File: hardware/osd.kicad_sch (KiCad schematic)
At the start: 21 parts, among them U10 COS8051SOT, U11 TLV7031DPWR, U18 SN74LVC1G3157DTBR

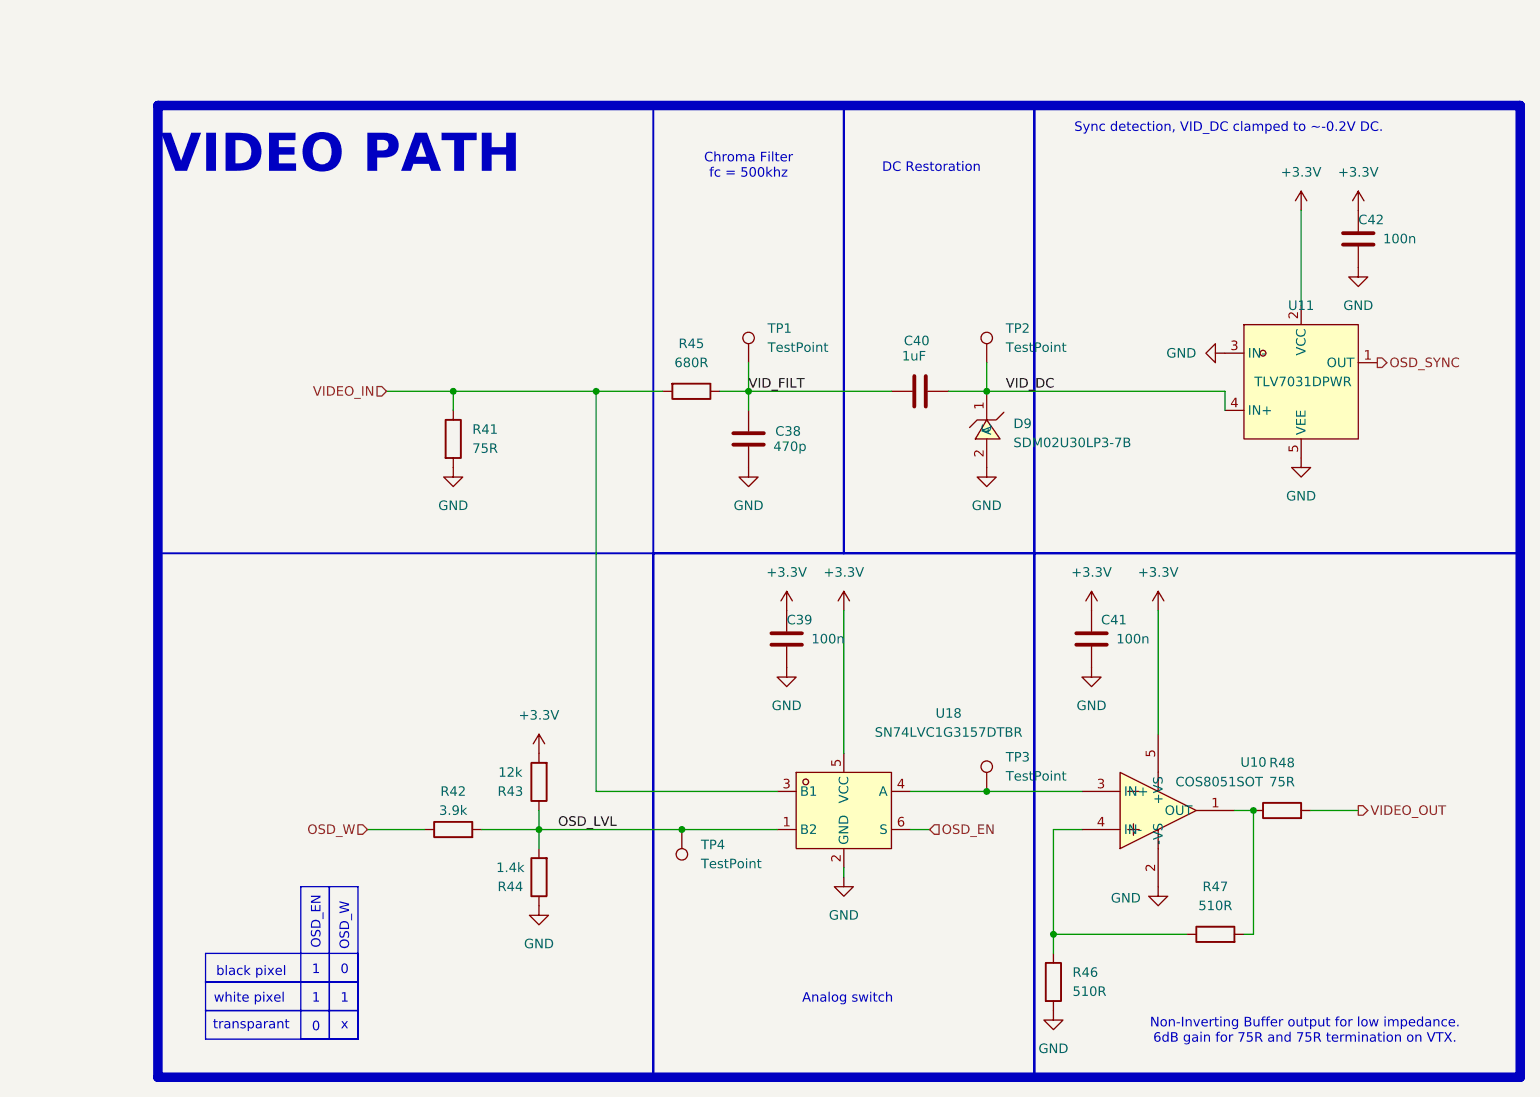
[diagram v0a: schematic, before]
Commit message: routing
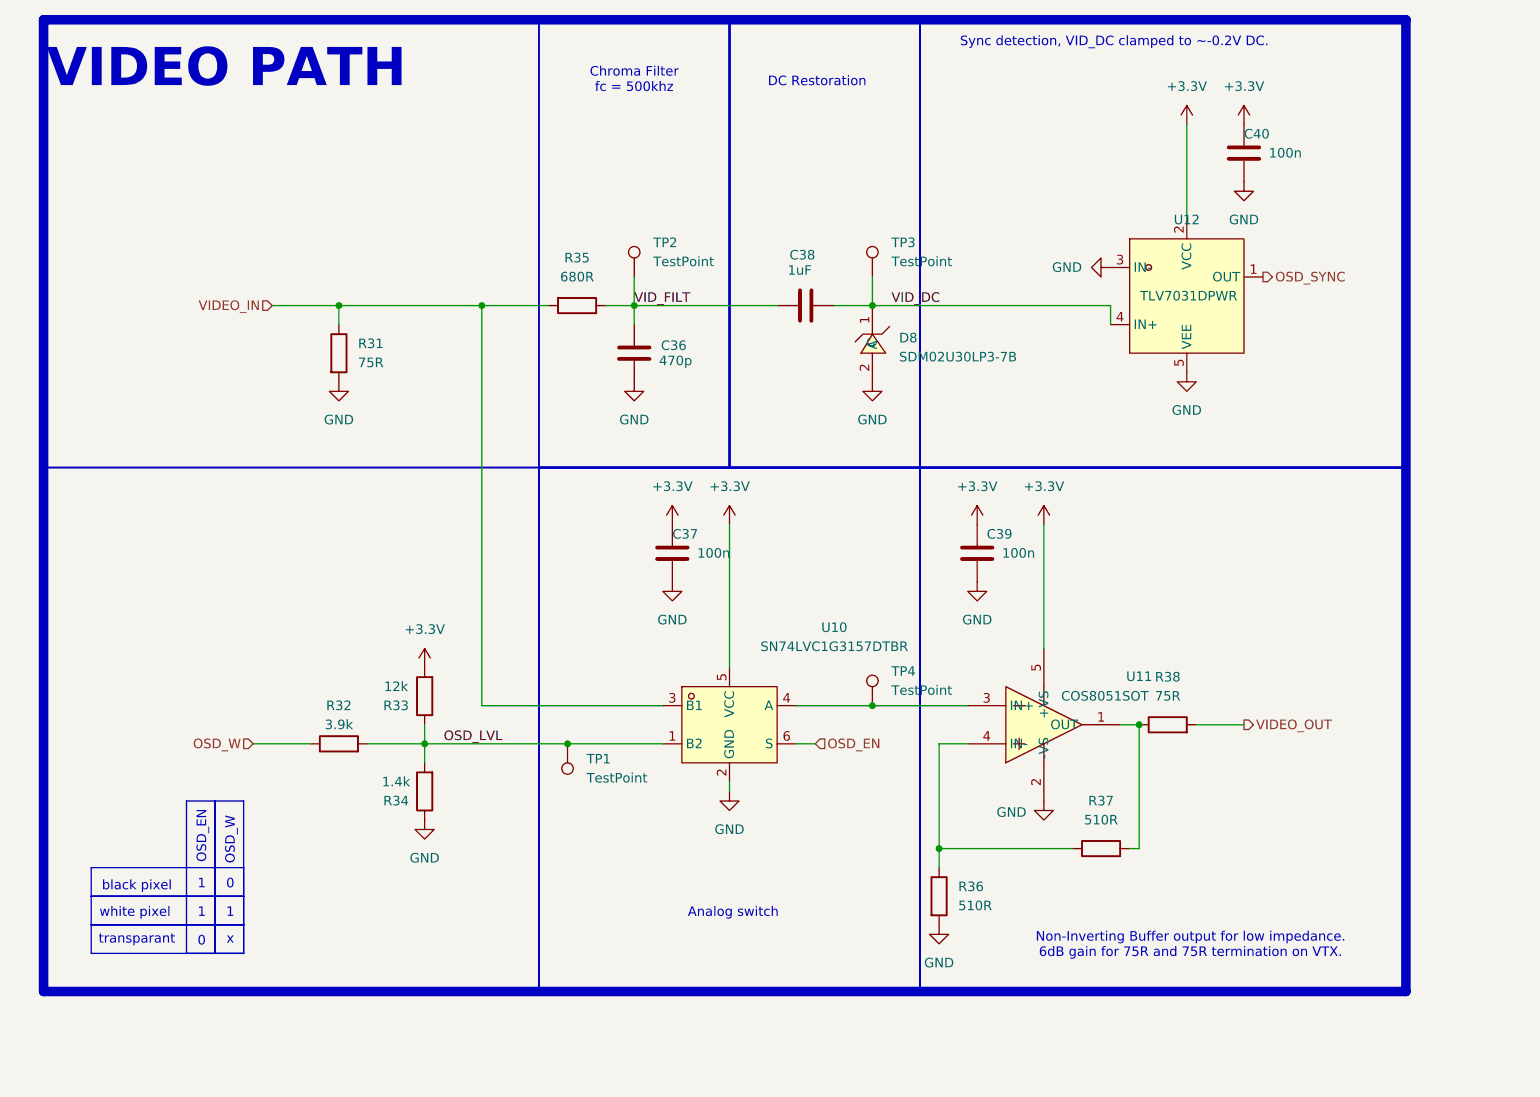
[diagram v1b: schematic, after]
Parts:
- removed C41, C42: 100n, Capacitor_SMD:C_0201_0603Metric, symbol Device:C
- removed D9: SDM02U30LP3-7B, lib:X3-DFN0603-2_L0.6-W0.3-RD, symbol lib:SDM02U30LP3-7B
- removed R41, R48: 75R, Resistor_SMD:R_0201_0603Metric, symbol Device:R
- removed R42: 3.9k, Resistor_SMD:R_0201_0603Metric, symbol Device:R
- removed R43: 12k, Resistor_SMD:R_0201_0603Metric, symbol Device:R
- removed R44: 1.4k, Resistor_SMD:R_0201_0603Metric, symbol Device:R
- removed R45: 680R, Resistor_SMD:R_0201_0603Metric, symbol Device:R
- removed R46, R47: 510R, Resistor_SMD:R_0201_0603Metric, symbol Device:R
- removed U10: COS8051SOT, lib:SOT-23-5_L3.0-W1.7-P0.95-LS2.8-BR, symbol lib:COS8051SOT
- removed U11: TLV7031DPWR, lib:X2SON-4_L0.8-W0.8-P0.48-TL-A, symbol lib:TLV7031DPWR
- removed U18: SN74LVC1G3157DTBR, lib:X2SON-6_L1.0-W0.8-BL, symbol lib:SN74LVC1G3157DTBR
- added C36: 470p, Capacitor_SMD:C_0201_0603Metric, symbol Device:C
- added C37: 100n, Capacitor_SMD:C_0201_0603Metric, symbol Device:C
- added D8: SDM02U30LP3-7B, lib:X3-DFN0603-2_L0.6-W0.3-RD, symbol lib:SDM02U30LP3-7B
- added R31, R38: 75R, Resistor_SMD:R_0201_0603Metric, symbol Device:R
- added R32: 3.9k, Resistor_SMD:R_0201_0603Metric, symbol Device:R
- added R33: 12k, Resistor_SMD:R_0201_0603Metric, symbol Device:R
- added R34: 1.4k, Resistor_SMD:R_0201_0603Metric, symbol Device:R
- added R35: 680R, Resistor_SMD:R_0201_0603Metric, symbol Device:R
- added R36, R37: 510R, Resistor_SMD:R_0201_0603Metric, symbol Device:R
- added U10: SN74LVC1G3157DTBR, lib:X2SON-6_L1.0-W0.8-BL, symbol lib:SN74LVC1G3157DTBR
- added U11: COS8051SOT, lib:SOT-23-5_L3.0-W1.7-P0.95-LS2.8-BR, symbol lib:COS8051SOT
- added U12: TLV7031DPWR, lib:X2SON-4_L0.8-W0.8-P0.48-TL-A, symbol lib:TLV7031DPWR
- C38: value 470p -> 1uF; footprint Capacitor_SMD:C_0201_0603Metric -> Capacitor_SMD:C_0402_1005Metric; LCSC C526944 -> C52923; MPN CC0201JRX7R9BB471 -> CL05A105KA5NQNC; Manufacturer YAGEO -> Samsung Electro-Mechanics
- C40: value 1uF -> 100n; footprint Capacitor_SMD:C_0402_1005Metric -> Capacitor_SMD:C_0201_0603Metric; LCSC C52923 -> C76928; MPN CL05A105KA5NQNC -> GRM033R60J104KE19D; Manufacturer Samsung Electro-Mechanics -> Murata Electronics
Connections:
- net +3.3V: now also C40.1, C37.1, R33.2, U10.5 (VCC), U11.5 (+VS), U12.2 (VCC)
- net GND: now also C40.2, C36.2, C37.2, D8.2 (A), R31.2, R34.1, R36.2, U10.2 (GND), U11.2 (-VS), U12.3 (IN-), U12.5 (VEE); no longer C38.2
- net OSD_EN: now also U10.6 (S)
- net OSD_LVL: now also TP1.1, R32.2, R33.1, R34.2, U10.1 (B2); no longer TP4.1
- net OSD_SYNC: now also U12.1 (OUT)
- net OSD_W: now also R32.1
- net VIDEO_IN: now also R31.1, R35.2, U10.3 (B1)
- net VIDEO_OUT: now also R38.2
- net VID_DC: now also C38.2, TP3.1, D8.1 (C), U12.4 (IN+); no longer C40.2, TP2.1
- net VID_FILT: now also TP2.1, C36.1, R35.1; no longer C40.1, TP1.1
- new net: TP4.1, U10.4 (A), U11.3 (IN+)
- new net: R37.2, R38.1, U11.1 (OUT)
- new net: R36.1, R37.1, U11.4 (IN-)
